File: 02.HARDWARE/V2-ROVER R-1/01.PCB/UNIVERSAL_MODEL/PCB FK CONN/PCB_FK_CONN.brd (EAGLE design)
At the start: 23.3 x 23.5 mm, 0 parts

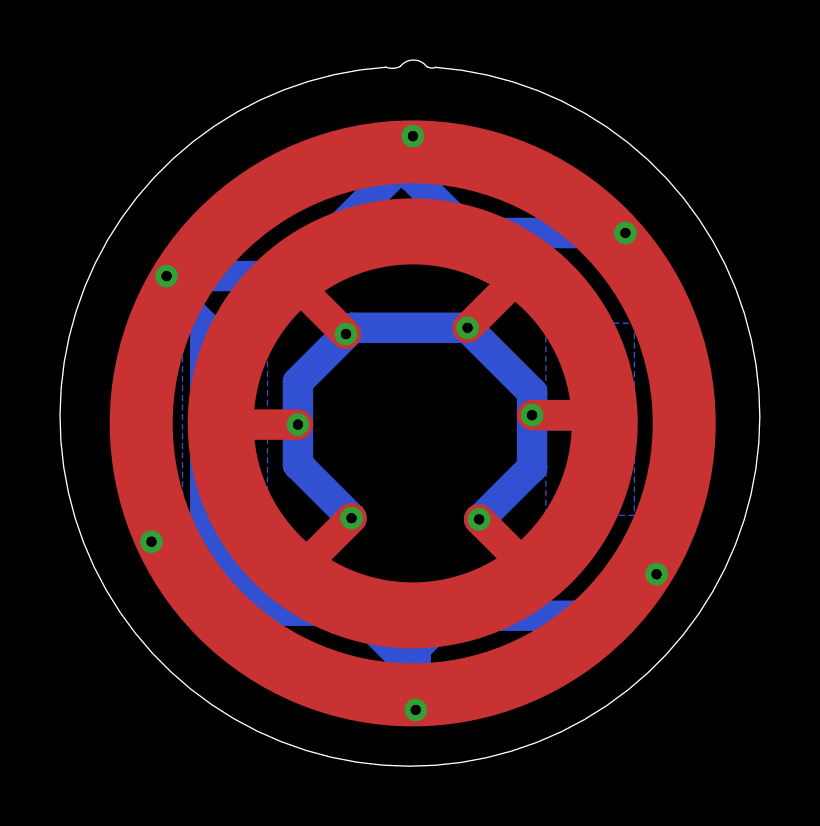
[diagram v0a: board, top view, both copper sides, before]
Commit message: Pedido y actualizacion
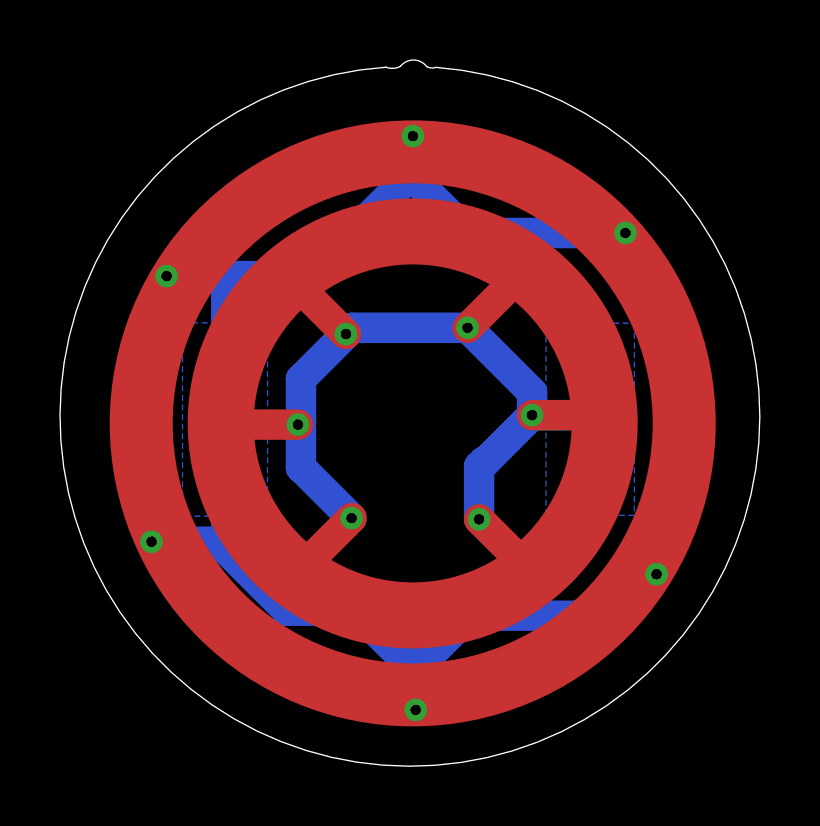
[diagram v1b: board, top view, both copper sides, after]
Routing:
- net A: track 53.9 -> 56.1 mm
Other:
- board text added: ""I love it when a plan comes together""
- board text removed: "***"
- board text removed: "F Irons"
- board text removed: "K"
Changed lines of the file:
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@@
 <grid distance="0.1" unitdist="mm" unit="mm" style="lines" multiple="1" display="yes" altdistance="5" altunitdist="mil" altunit="mil"/>
 <layers>
-<layer number="1" name="Top" color="4" fill="1" visible="no" active="yes"/>
-<layer number="16" name="Bottom" color="1" fill="1" visible="yes" active="yes"/>
+<layer number="1" name="Top" color="4" fill="1" visible="yes" active="yes"/>
+<layer number="16" name="Bottom" color="1" fill="1" visible="no" active="yes"/>
 <layer number="17" name="Pads" color="2" fill="1" visible="yes" active="yes"/>
 <layer number="18" name="Vias" color="2" fill="1" visible="yes" active="yes"/>
 <layer number="19" name="Unrouted" color="6" fill="1" visible="yes" active="yes"/>
 <layer number="20" name="Dimension" color="24" fill="1" visible="yes" active="yes"/>
-<layer number="21" name="tPlace" color="7" fill="1" visible="no" active="yes"/>
-<layer number="22" name="bPlace" color="7" fill="1" visible="yes" active="yes"/>
-<layer number="23" name="tOrigins" color="15" fill="1" visible="no" active="yes"/>
-<layer number="24" name="bOrigins" color="15" fill="1" visible="yes" active="yes"/>
-<layer number="25" name="tNames" color="7" fill="1" visible="no" active="yes"/>
-<layer number="26" name="bNames" color="7" fill="1" visible="yes" active="yes"/>
+<layer number="21" name="tPlace" color="7" fill="1" visible="yes" active="yes"/>
+<layer number="22" name="bPlace" color="7" fill="1" visible="no" active="yes"/>
+<layer number="23" name="tOrigins" color="15" fill="1" visible="yes" active="yes"/>
+<layer number="24" name="bOrigins" color="15" fill="1" visible="no" active="yes"/>
+<layer number="25" name="tNames" color="7" fill="1" visible="yes" active="yes"/>
+<layer number="26" name="bNames" color="7" fill="1" visible="no" active="yes"/>
 <layer number="27" name="tValues" color="7" fill="1" visible="no" active="yes"/>
 <layer number="28" name="bValues" color="7" fill="1" visible="no" active="yes"/>
@@
 <layer number="37" name="tTest" color="7" fill="1" visible="no" active="yes"/>
 <layer number="38" name="bTest" color="7" fill="1" visible="no" active="yes"/>
-<layer number="39" name="tKeepout" color="4" fill="11" visible="no" active="yes"/>
-<layer number="40" name="bKeepout" color="1" fill="11" visible="yes" active="yes"/>
-<layer number="41" name="tRestrict" color="4" fill="10" visible="no" active="yes"/>
-<layer number="42" name="bRestrict" color="1" fill="10" visible="yes" active="yes"/>
+<layer number="39" name="tKeepout" color="4" fill="11" visible="yes" active="yes"/>
+<layer number="40" name="bKeepout" color="1" fill="11" visible="no" active="yes"/>
+<layer number="41" name="tRestrict" color="4" fill="10" visible="yes" active="yes"/>
+<layer number="42" name="bRestrict" color="1" fill="10" visible="no" active="yes"/>
 <layer number="43" name="vRestrict" color="2" fill="10" visible="no" active="yes"/>
 <layer number="44" name="Drills" color="7" fill="1" visible="no" active="yes"/>
@@
 <layer number="49" name="Reference" color="7" fill="1" visible="no" active="yes"/>
 <layer number="50" name="dxf" color="7" fill="1" visible="no" active="no"/>
-<layer number="51" name="tDocu" color="7" fill="1" visible="no" active="yes"/>
-<layer number="52" name="bDocu" color="7" fill="1" visible="yes" active="yes"/>
+<layer number="51" name="tDocu" color="7" fill="1" visible="yes" active="yes"/>
+<layer number="52" name="bDocu" color="7" fill="1" visible="no" active="yes"/>
 <layer number="53" name="tGND_GNDA" color="7" fill="9" visible="no" active="no"/>
 <layer number="54" name="bGND_GNDA" color="1" fill="9" visible="no" active="no"/>
@@
 <text x="75" y="63.5" size="1.016" layer="22" font="vector" rot="MR0">FK_CONN
 v1-Feb24</text>
-<text x="73" y="69.85" size="1.016" layer="22" font="vector" rot="MR0">F
-Irons</text>
-<text x="72.5" y="71.4" size="0.1" layer="22" font="vector" rot="MR0">***</text>
-<text x="71.9" y="71.37" size="1.016" layer="22" font="vector" rot="MR0">K</text>
+<text x="75.8" y="68.45" size="1.016" layer="22" font="vector" rot="MR0">"I love it
+when a plan
+comes
+together"</text>
 </plain>
 <attributes>
@@
 <wire x1="75.979" y1="71.274" x2="78.679" y2="71.274" width="1.016" layer="16"/>
 <wire x1="78.679" y1="71.274" x2="78.732" y2="71.327" width="1.016" layer="16"/>
-<wire x1="69.962" y1="67.842" x2="68.175" y2="69.629" width="1.016" layer="16"/>
-<wire x1="68.175" y1="69.629" x2="68.175" y2="70.96" width="1.016" layer="16"/>
-<wire x1="68.175" y1="70.96" x2="68.175" y2="72.379" width="1.016" layer="16"/>
-<wire x1="68.175" y1="72.379" x2="69.774" y2="73.978" width="1.016" layer="16"/>
+<wire x1="69.962" y1="67.842" x2="68.275" y2="69.529" width="1.016" layer="16"/>
+<wire x1="68.275" y1="70.86" x2="68.275" y2="69.529" width="1.016" layer="16"/>
+<wire x1="68.275" y1="70.86" x2="68.175" y2="70.96" width="1.016" layer="16"/>
+<wire x1="68.175" y1="70.96" x2="68.275" y2="71.06" width="1.016" layer="16"/>
+<wire x1="68.275" y1="72.479" x2="68.275" y2="71.06" width="1.016" layer="16"/>
+<wire x1="68.275" y1="72.479" x2="69.774" y2="73.978" width="1.016" layer="16"/>
 <wire x1="69.774" y1="73.978" x2="69.981" y2="74.185" width="1.016" layer="16"/>
 <wire x1="69.981" y1="74.185" x2="73.829" y2="74.185" width="1.016" layer="16"/>
 <wire x1="73.829" y1="74.185" x2="75.979" y2="72.035" width="1.016" layer="16"/>
 <wire x1="75.979" y1="72.035" x2="75.979" y2="71.274" width="1.016" layer="16"/>
-<wire x1="75.979" y1="69.53" x2="74.251" y2="67.802" width="1.016" layer="16"/>
-<wire x1="74.214" y1="67.802" x2="74.251" y2="67.802" width="1.016" layer="16"/>
-<wire x1="75.979" y1="69.53" x2="75.979" y2="71.274" width="1.016" layer="16"/>
+<wire x1="74.214" y1="67.802" x2="74.214" y2="69.565" width="1.016" layer="16"/>
+<wire x1="74.379" y1="69.73" x2="74.214" y2="69.565" width="1.016" layer="16"/>
+<wire x1="74.435" y1="69.73" x2="75.979" y2="71.274" width="1.016" layer="16"/>
+<wire x1="74.435" y1="69.73" x2="74.379" y2="69.73" width="1.016" layer="16"/>
 <wire x1="73.829" y1="74.185" x2="75.51" y2="75.866" width="1.016" layer="1"/>
 <wire x1="75.51" y1="75.866" x2="75.51" y2="75.89" width="1.016" layer="1"/>
@@
 <via x="72.101" y="61.45" extent="1-16" drill="0.35"/>
 <via x="63.294" y="67.055" extent="1-16" drill="0.35"/>
-<wire x1="63.294" y1="67.055" x2="65.086" y2="67.055" width="1.016" layer="16"/>
-<wire x1="63.796" y1="75.91" x2="63.796" y2="75.513" width="1.016" layer="16"/>
-<wire x1="65.086" y1="74.223" x2="63.796" y2="75.513" width="1.016" layer="16"/>
-<wire x1="65.086" y1="74.223" x2="65.086" y2="67.055" width="1.016" layer="16"/>
-<wire x1="72.006" y1="80.575" x2="72.006" y2="79.96" width="1.016" layer="16"/>
-<wire x1="72.006" y1="79.96" x2="67.956" y2="75.91" width="1.016" layer="16"/>
-<wire x1="63.796" y1="75.91" x2="67.956" y2="75.91" width="1.016" layer="16"/>
+<wire x1="65.786" y1="66.955" x2="63.394" y2="66.955" width="1.016" layer="16"/>
+<wire x1="63.294" y1="67.055" x2="63.394" y2="66.955" width="1.016" layer="16"/>
+<wire x1="63.796" y1="75.91" x2="65.786" y2="75.91" width="1.016" layer="16"/>
+<wire x1="65.786" y1="75.91" x2="65.786" y2="66.955" width="1.016" layer="16"/>
+<wire x1="72.006" y1="80.575" x2="72.006" y2="79.36" width="1.016" layer="16"/>
+<wire x1="72.006" y1="79.36" x2="68.556" y2="75.91" width="1.016" layer="16"/>
+<wire x1="63.796" y1="75.91" x2="68.556" y2="75.91" width="1.016" layer="16"/>
 <wire x1="73.86" y1="77.347" x2="79.091" y2="77.347" width="1.016" layer="16"/>
 <wire x1="72.006" y1="80.575" x2="72.006" y2="79.201" width="1.016" layer="16"/>
 <wire x1="73.86" y1="77.347" x2="72.006" y2="79.201" width="1.016" layer="16"/>
 <wire x1="80.13" y1="65.973" x2="78.748" y2="64.591" width="1.016" layer="16"/>
-<wire x1="78.748" y1="64.591" x2="73.18" y2="64.591" width="1.016" layer="16"/>
-<wire x1="73.18" y1="64.591" x2="72.101" y2="63.512" width="1.016" layer="16"/>
-<wire x1="72.101" y1="63.512" x2="72.101" y2="61.45" width="1.016" layer="16"/>
+<wire x1="78.748" y1="64.591" x2="73.88" y2="64.591" width="1.016" layer="16"/>
+<wire x1="73.88" y1="64.591" x2="72.101" y2="62.812" width="1.016" layer="16"/>
+<wire x1="72.101" y1="62.812" x2="72.101" y2="61.45" width="1.016" layer="16"/>
 <wire x1="72.101" y1="61.45" x2="72.101" y2="62.749" width="1.016" layer="16"/>
 <wire x1="72.101" y1="62.749" x2="70.09" y2="64.76" width="1.016" layer="16"/>
-<wire x1="70.09" y1="64.76" x2="67.413" y2="64.76" width="1.016" layer="16"/>
-<wire x1="67.413" y1="64.76" x2="65.118" y2="67.055" width="1.016" layer="16"/>
-<wire x1="65.118" y1="67.055" x2="63.294" y2="67.055" width="1.016" layer="16"/>
+<wire x1="70.09" y1="64.76" x2="67.813" y2="64.76" width="1.016" layer="16"/>
+<wire x1="67.813" y1="64.76" x2="65.518" y2="67.055" width="1.016" layer="16"/>
+<wire x1="65.518" y1="67.055" x2="63.294" y2="67.055" width="1.016" layer="16"/>
 </signal>
 </signals>
